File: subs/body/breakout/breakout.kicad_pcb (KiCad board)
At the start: 2 copper layers, 37.2 x 27.5 mm, 27 parts, among them P1 CONN_SRV_CAM, P10 CONN_UART, P11 CONN_I2C, P12 CONN_FAN, P14 CONN_IR, P15 CONN_STEP, P16 CONN_EP_VCC, P17 CONN_BTN, P18 CONN3, P19 CONN4, P2 CONN_SRV_LOCK, P21 CONN1, P22 CONN2, P3 CONN_SRV_BRAKE, P4 CONN_SRV_FOOT, P5 CONN_VCC, P6 CONN_STEP_STOP, P7 CONN_LED, P8 CONN_BAT_INT, P9 CONN_EP_UART, U1 MCP23017, U2 TMP101

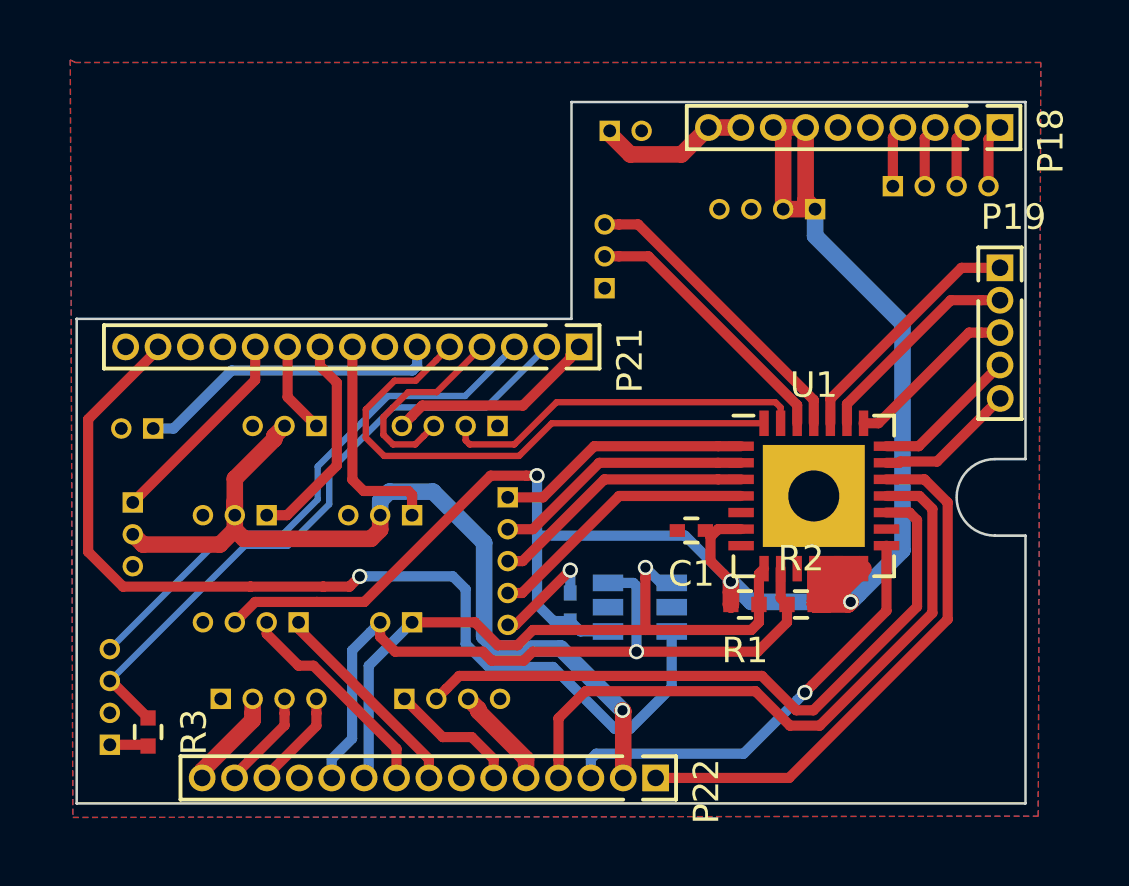
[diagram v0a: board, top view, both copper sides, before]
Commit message: In progress, commit for backup
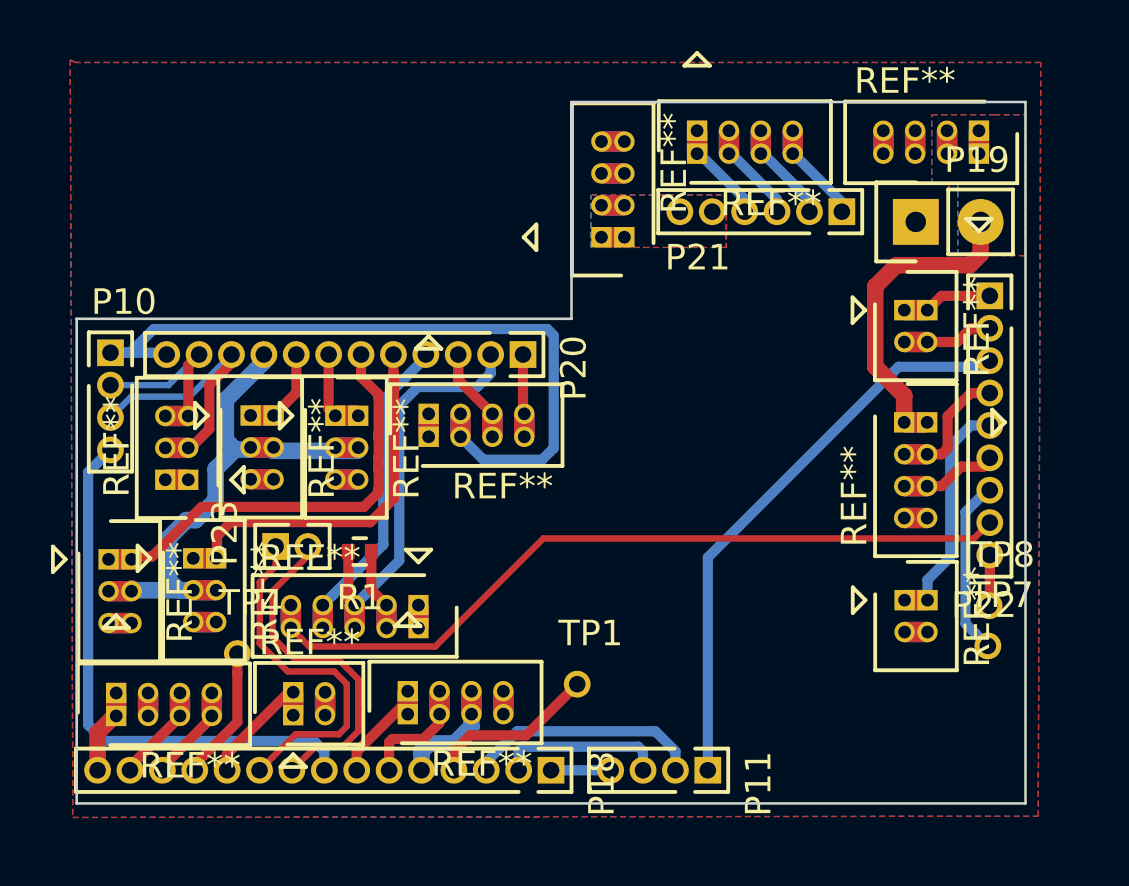
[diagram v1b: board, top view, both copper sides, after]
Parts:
- removed C1, C2: 100nF, Capacitors_SMD:C_0402
- removed R2: 10K, Resistors_SMD:R_0402_Handsoldering
- removed R3: 100K, Resistors_SMD:R_0402_Handsoldering
- removed U1: MCP23017, Housings_DFN_QFN:QFN-28-1EP-NPTH_6x6mm_Pitch0.65mm
- removed U2: TMP101, TO_SOT_Packages_SMD:SOT-23-6_Handsoldering
- added P13: CONN_LED, Connectors_Molex:Molex_PicoBlade_53047-0410_DoubleSide, B.Cu at (63.4, 120.2)
- added P20: CONN1, Socket_Strips:Socket_Strip_Straight_1x12_Pitch1.27mm, F.Cu at (79.3, 106.9)
- added P23: CONN_I2C0, Pin_Headers:Pin_Header_Straight_1x02_Pitch1.27mm, F.Cu at (69.6, 114.4)
- added P24: CONN_I2C1, Connectors_Molex:Molex_PicoBlade_53047-0210_DoubleSide, B.Cu at (95.2, 105.2)
- added TP1: TEST_1P, Pin_Headers:Pin_Header_Straight_1x01_Pitch1.27mm, F.Cu at (81.4, 119.8)
- added TP4: TEST_1P, Pin_Headers:Pin_Header_Straight_1x01_Pitch1.27mm, F.Cu at (68.1, 118.6)
- added TP7: TEST_1P, Pin_Headers:Pin_Header_Straight_1x01_Pitch1.27mm, F.Cu at (97.5, 118.3)
- added TP8: TEST_1P, Pin_Headers:Pin_Header_Straight_1x01_Pitch1.27mm, F.Cu at (97.6, 116.8)
- P1: value CONN_SRV_CAM -> CONN_UART; footprint Connectors_Molex:Molex_PicoBlade_53047-0310 -> Connectors_Molex:Molex_PicoBlade_53047-0510_DoubleSide
- P10: value CONN_UART -> CONN_SPI0; footprint Connectors_Molex:Molex_PicoBlade_53047-0410 -> Pin_Headers:Pin_Header_Straight_1x04_Pitch1.27mm; moved to F.Cu
- P11: value CONN_I2C -> CONN_SPI1; footprint Connectors_Molex:Molex_PicoBlade_53047-0210 -> Pin_Headers:Pin_Header_Straight_1x04_Pitch1.27mm; moved to F.Cu
- P12: value CONN_FAN -> CONN_BTN; footprint Connectors_Molex:Molex_PicoBlade_53047-0410 -> Connectors_Molex:Molex_PicoBlade_53047-0210_DoubleSide
- P14: value CONN_IR -> CONN_VCC; footprint Connectors_Molex:Molex_PicoBlade_53047-0410 -> Connectors_Molex:Molex_PicoBlade_53047-0410_DoubleSide
- P15, P9: footprint Connectors_Molex:Molex_PicoBlade_53047-0410 -> Connectors_Molex:Molex_PicoBlade_53047-0410_DoubleSide
- P16: footprint Connectors_Molex:Molex_PicoBlade_53047-0210 -> Connectors_Molex:Molex_PicoBlade_53047-0410_DoubleSide
- P17: value CONN_BTN -> CONN_IR; footprint Connectors_Molex:Molex_PicoBlade_53047-0510 -> Connectors_Molex:Molex_PicoBlade_53047-0410_DoubleSide
- P18: value CONN3 -> CONN2; footprint Pin_Headers:Pin_Header_Straight_1x10_Pitch1.27mm -> Socket_Strips:Socket_Strip_Straight_1x15_Pitch1.27mm
- P19: value CONN4 -> CONN_VCC; footprint Pin_Headers:Pin_Header_Straight_1x05_Pitch1.27mm -> Socket_Strips:Socket_Strip_Straight_1x02
- P2: value CONN_SRV_LOCK -> CONN_SRV_CAM; footprint Connectors_Molex:Molex_PicoBlade_53047-0310 -> Connectors_Molex:Molex_PicoBlade_53047-0310_DoubleSide
- P21: value CONN1 -> CONN3; footprint Pin_Headers:Pin_Header_Straight_1x15_Pitch1.27mm -> Socket_Strips:Socket_Strip_Straight_1x06_Pitch1.27mm
- P22: value CONN2 -> CONN4; footprint Pin_Headers:Pin_Header_Straight_1x15_Pitch1.27mm -> Socket_Strips:Socket_Strip_Straight_1x09_Pitch1.27mm
- P3: value CONN_SRV_BRAKE -> CONN_SRV_LOCK; footprint Connectors_Molex:Molex_PicoBlade_53047-0310 -> Connectors_Molex:Molex_PicoBlade_53047-0310_DoubleSide
- P4: value CONN_SRV_FOOT -> CONN_SRV_BRAKE; footprint Connectors_Molex:Molex_PicoBlade_53047-0310 -> Connectors_Molex:Molex_PicoBlade_53047-0310_DoubleSide
- P5: value CONN_VCC -> CONN_SRV_FOOT; footprint Connectors_Molex:Molex_PicoBlade_53047-0410 -> Connectors_Molex:Molex_PicoBlade_53047-0310_DoubleSide
- P6: footprint Connectors_Molex:Molex_PicoBlade_53047-0310 -> Connectors_Molex:Molex_PicoBlade_53047-0310_DoubleSide
- P7: value CONN_LED -> CONN_FAN; footprint Connectors_Molex:Molex_PicoBlade_53047-0410 -> Connectors_Molex:Molex_PicoBlade_53047-0410_DoubleSide
- P8: footprint Connectors_Molex:Molex_PicoBlade_53047-0210 -> Connectors_Molex:Molex_PicoBlade_53047-0210_DoubleSide
- R1: value 10K -> 100K; footprint Resistors_SMD:R_0402_Handsoldering -> Resistors_SMD:R_0402
- moved P14 32.4 mm to (97.2, 99.0)
- moved P8 31.1 mm to (95.2, 116.5), turned to 270 degrees
- moved P18 30.7 mm to (80.4, 123.2)
- moved P5 30.1 mm to (64.0, 114.9), turned to 270 degrees
- moved P22 23.0 mm to (97.6, 104.6), turned to 0 degrees
- moved P6 18.8 mm to (65.3, 111.8)
- moved P17 16.7 mm to (95.1, 109.6)
- moved P10 15.4 mm to (63.1, 106.8), turned to 0 degrees
- moved R1 15.2 mm to (72.9, 114.6)
- moved P11 13.0 mm to (86.5, 123.2), turned to 270 degrees
- moved P21 11.6 mm to (91.8, 101.3)
- moved P15 7.98 mm to (86.1, 98.1)
- moved P7 7.34 mm to (74.8, 120.1)
- moved P4 5.30 mm to (72.8, 109.3), turned to 270 degrees
- moved P1 4.43 mm to (75.2, 117.6)
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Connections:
- P1 pad 1: /SRV_CAM -> GND
- P1 pad 2: /SRV_VOUT -> /UART_VCC
- P1 pad 3: GND -> /UART_TX
- P10 pad 1: /UART_VCC -> /SCK0/FRAME_STOP
- P10 pad 2: GND -> /MISO0/STEP_STOP2
- P10 pad 3: /UART_TX -> /MOSI0/STEP_STOP1
- P10 pad 4: /UART_RX -> /~RESET0
- P11 pad 1: /SCL -> /~RESET1
- P11 pad 2: /SDA -> /BAT2_CTL/SCK1
- P12 pad 1: /MOSI/FAN_PWM -> /BUTTON
- P12 pad 2: /FAN_TACHO -> GND
- P14 pad 1: /IR_RX -> VCC
- P14 pad 2: /IR_TX -> VCC
- P14 pad 3: VCC -> GND
- P16 pad 2: GND -> /EP_VCC
- P17 pad 1: /BTN1 -> VCC
- P17 pad 2: /BTN2 -> /IR_TX
- P17 pad 3: /BTN3 -> /IR_RX
- P17 pad 4: /BTN4 -> GND
- P18 pad 1: /STEP_A1 -> /CHG2_STAT/MISO1
- P18 pad 10: /EP_VCC -> /SDA0
- P18 pad 2: /STEP_A2 -> /CHG2_CTL/MOSI1
- P18 pad 3: /STEP_B2 -> /BAT2_CTL/SCK1
- P18 pad 4: /STEP_B1 -> /TMP_INT0
- P18 pad 5: GND -> /FAN_VOUT
- P18 pad 6: GND -> /FAN_TACHO
- P18 pad 7: VCC -> /FAN_PWM
- P18 pad 8: VCC -> /~RESET0
- P18 pad 9: /EP_VCC -> /SCL0
- P19 pad 1: /STEP_DIR -> GND
- P19 pad 2: /~STEP_SLP -> VCC
- P2 pad 1: /SCK/SRV_LOCK -> /SRV_CAM
- P21 pad 1: /EP_RXD -> /STEP_A1
- P21 pad 2: /UART_TX -> /STEP_A2
- P21 pad 3: /UART_RX -> /STEP_B2
- P21 pad 4: /EP_TXD -> /STEP_B1
- P21 pad 5: /LED_EN -> /EP_VCC
- P21 pad 6: /BAT_INT -> /EP_VCC
- P22 pad 1: /SRV_EN -> /SDA1
- P22 pad 2: /SRV_VOUT -> /SCL1
- P22 pad 3: /INT -> /~RESET1
- P22 pad 4: /FAN_EN -> /IR_TX
- P22 pad 5: /FAN_VOUT -> /BAT_INT
- P22 pad 6: /MOSI/FAN_PWM -> /IR_RX
- P22 pad 7: GND -> /PWR_INT
- P22 pad 8: /IR_RX -> /HOST_INT
- P22 pad 9: /IR_TX -> /TMP_INT1
- P3 pad 1: /MISO/SRV_BRAKE -> /SRV_LOCK
- P4 pad 1: /~SS~/SRV_FOOT -> /SRV_BRAKE
- P5 pad 1: VCC -> /SRV_FOOT
- P5 pad 2: VCC -> /SRV_VOUT
- P6 pad 2: /STEP_STOP2 -> /MOSI0/STEP_STOP1
- P6 pad 3: /STEP_STOP1 -> /MISO0/STEP_STOP2
- P7 pad 1: GND -> /FAN_PWM
- P7 pad 2: /LED_VOUT -> /FAN_TACHO
- P7 pad 3: /LED_DAT -> /FAN_VOUT
- P7 pad 4: /LED_CLK -> GND
- P9 pad 2: /FRAME_STOP -> /SCK0/FRAME_STOP
- R1 pad 1: /SCL -> /UART_VCC
- R1 pad 2: VCC -> /UART_TX
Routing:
- net VCC: track 76.1 -> 11.7 mm, vias 3 -> 0
- net /A6: track 39.4 -> 0.00 mm, vias 1 -> 0
- net /HOST_INT: track 0.00 -> 30.6 mm
- net /SDA: track 30.4 -> 0.00 mm, vias 1 -> 0
- net /SCK0/FRAME_STOP: track 0.00 -> 29.6 mm
- net /SCL: track 27.1 -> 0.00 mm, vias 1 -> 0
- net /FAN_EN: track 25.9 -> 0.00 mm
- net /~RESET1: track 0.00 -> 22.6 mm
- net /LED_EN: track 21.8 -> 0.00 mm
- net /~RESET0: track 0.00 -> 21.6 mm
- net /FAN_TACHO: track 26.2 -> 4.71 mm
- net /SRV_EN: track 21.4 -> 0.00 mm
- net /INT: track 17.3 -> 0.00 mm, vias 1 -> 0
- net /SRV_FOOT: track 0.00 -> 16.4 mm
- net /SRV_VOUT: track 35.0 -> 20.1 mm, vias 1 -> 0
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- added copper zone on B.Cu, net /EP_VCC
- added copper zone on F.Cu, net /EP_VCC
- added copper zone on B.Cu, net VCC
- added copper zone on F.Cu, net VCC
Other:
- outline, holes or cut-outs redrawn

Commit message: Major modification of body board and companions
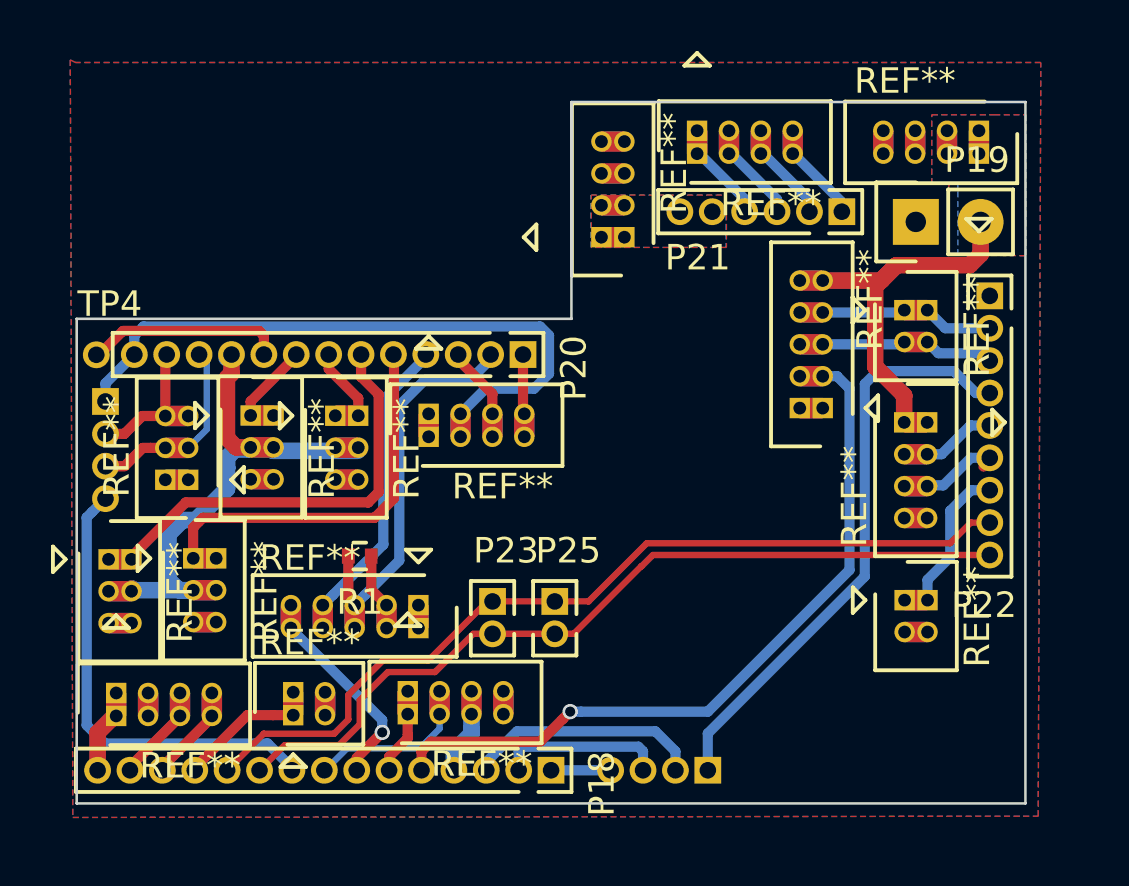
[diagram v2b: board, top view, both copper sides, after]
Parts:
- removed TP1, TP7, TP8: TEST_1P, Pin_Headers:Pin_Header_Straight_1x01_Pitch1.27mm
- added P25: CONN_I2C2, Pin_Headers:Pin_Header_Straight_1x02_Pitch1.27mm, F.Cu at (80.5, 116.6)
- added P26: CONN_TMP, Connectors_Molex:Molex_PicoBlade_53047-0510_DoubleSide, B.Cu at (90.2, 109.0)
- P10, P11: moved to B.Cu
- P20: footprint Socket_Strips:Socket_Strip_Straight_1x12_Pitch1.27mm -> Socket_Strips:Socket_Strip_Straight_1x13_Pitch1.27mm
- moved TP4 13.0 mm to (62.6, 106.9)
- moved P23 8.77 mm to (78.1, 116.6), turned to 0 degrees
- moved P10 1.92 mm to (62.9, 108.7), turned to 180 degrees
- moved R1 0.17 mm to (72.9, 114.8)
- turned P11 to 90 degrees
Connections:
- P18 pad 10: /SDA0 -> /SCL0
- P18 pad 11: /BUTTON -> /SDA0
- P18 pad 12: /A2 -> /BUTTON
- P18 pad 4: /TMP_INT0 -> /FAN_VOUT
- P18 pad 5: /FAN_VOUT -> /TMP_INT
- P18 pad 6: /FAN_TACHO -> /FAN_PWM
- P18 pad 7: /FAN_PWM -> /HOST_INT
- P18 pad 8: /~RESET0 -> /FAN_TACHO
- P18 pad 9: /SCL0 -> /~RESET0
- P20 pad 10: /MOSI0/STEP_STOP1 -> /SRV_VOUT
- P20 pad 11: /MISO0/STEP_STOP2 -> /MOSI0/STEP_STOP1
- P20 pad 12: /SCK0/FRAME_STOP -> /MISO0/STEP_STOP2
- P20 pad 9: /SRV_VOUT -> /A2
- P22 pad 1: /SDA1 -> (no net)
- P22 pad 2: /SCL1 -> /SDA1
- P22 pad 3: /~RESET1 -> /SCL1
- P22 pad 4: /IR_TX -> /~RESET1
- P22 pad 5: /BAT_INT -> /IR_TX
- P22 pad 7: /PWR_INT -> /BAT_INT
- P22 pad 8: /HOST_INT -> /SDA0
- P22 pad 9: /TMP_INT1 -> /SCL0
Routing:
- net /TMP_INT: track 0.00 -> 28.8 mm, vias 0 -> 1
- net /HOST_INT: track 30.6 -> 8.37 mm, vias 0 -> 1
- net /SDA0: track 13.9 -> 34.3 mm
- net /SCL0: track 13.4 -> 32.5 mm
- net /PWR_INT: track 7.12 -> 0.00 mm
- net /TMP_INT0: track 6.67 -> 0.00 mm
- net /MOSI0/STEP_STOP1: track 11.1 -> 6.73 mm
- net VCC: track 11.7 -> 15.8 mm
- net /~RESET0: track 21.6 -> 18.0 mm
- net /SCK0/FRAME_STOP: track 29.6 -> 26.1 mm
- net /SCL1: track 2.75 -> 5.99 mm
- net /SDA1: track 2.76 -> 5.98 mm
- net /BAT_INT: track 8.30 -> 5.76 mm
- net /A2: track 5.27 -> 7.78 mm
- net /FAN_VOUT: track 4.56 -> 2.49 mm
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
